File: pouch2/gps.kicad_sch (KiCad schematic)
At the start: 4 parts

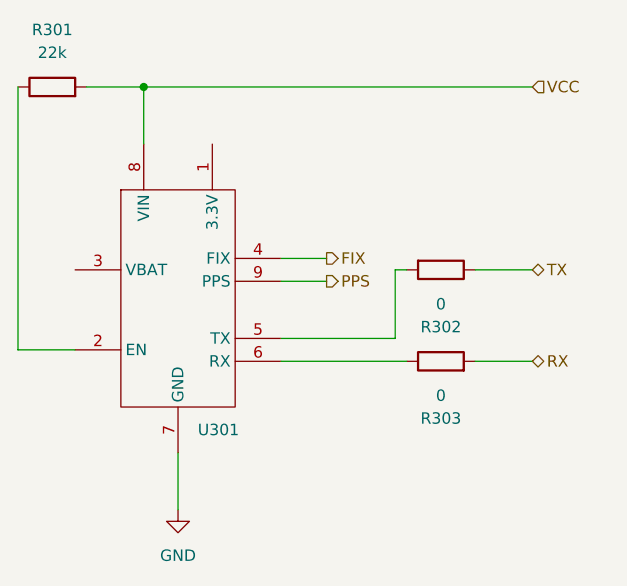
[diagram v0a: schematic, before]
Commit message: started routing
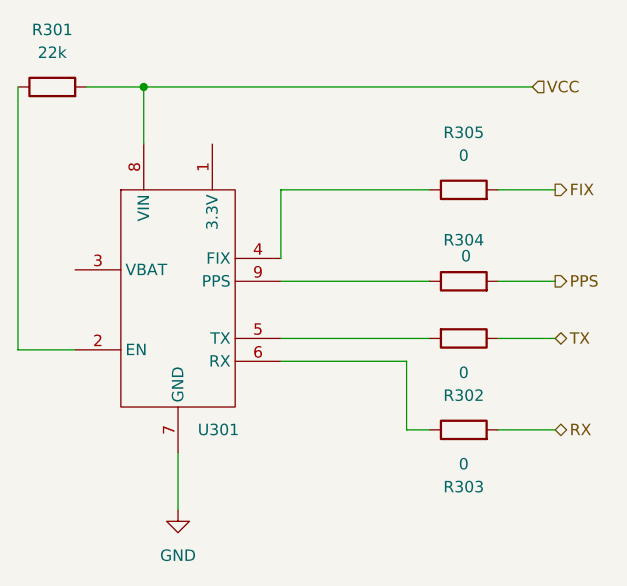
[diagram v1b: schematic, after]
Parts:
- added R304, R305: 0, Resistor_SMD:R_0805_2012Metric, symbol Device:R
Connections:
- net FIX: now also R305.2; no longer U301.4 (FIX)
- net PPS: now also R304.2; no longer U301.9 (PPS)
- new net: R304.1, U301.9 (PPS)
- new net: R305.1, U301.4 (FIX)
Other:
- moved on the sheet: R302, R303
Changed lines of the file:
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@@
-	(wire
-		(pts
-			(xy 182.88 67.31) (xy 182.88 74.93)
-		)
-		(stroke
-			(width 0)
-			(type default)
-		)
-	)
 	(wire
 		(pts
@@
 	(wire
 		(pts
+			(xy 184.15 77.47) (xy 170.18 77.47)
+		)
+		(stroke
+			(width 0)
+			(type default)
+		)
+	)
+	(wire
+		(pts
 			(xy 148.59 46.99) (xy 154.94 46.99)
 		)
@@
 	(wire
 		(pts
-			(xy 170.18 77.47) (xy 184.15 77.47)
-		)
-		(stroke
-			(width 0)
-			(type default)
-		)
-	)
-	(wire
-		(pts
-			(xy 170.18 68.58) (xy 175.26 68.58)
+			(xy 184.15 85.09) (xy 186.69 85.09)
+		)
+		(stroke
+			(width 0)
+			(type default)
+		)
+	)
+	(wire
+		(pts
+			(xy 170.18 68.58) (xy 186.69 68.58)
+		)
+		(stroke
+			(width 0)
+			(type default)
+		)
+	)
+	(wire
+		(pts
+			(xy 170.18 58.42) (xy 170.18 66.04)
 		)
 		(stroke
@@
 	(wire
 		(pts
-			(xy 198.12 67.31) (xy 191.77 67.31)
-		)
-		(stroke
-			(width 0)
-			(type default)
-		)
-	)
-	(wire
-		(pts
-			(xy 182.88 67.31) (xy 184.15 67.31)
-		)
-		(stroke
-			(width 0)
-			(type default)
-		)
-	)
-	(wire
-		(pts
-			(xy 170.18 66.04) (xy 175.26 66.04)
-		)
-		(stroke
-			(width 0)
-			(type default)
-		)
-	)
-	(wire
-		(pts
-			(xy 170.18 74.93) (xy 182.88 74.93)
-		)
-		(stroke
-			(width 0)
-			(type default)
-		)
-	)
-	(wire
-		(pts
-			(xy 198.12 77.47) (xy 191.77 77.47)
+			(xy 200.66 74.93) (xy 194.31 74.93)
+		)
+		(stroke
+			(width 0)
+			(type default)
+		)
+	)
+	(wire
+		(pts
+			(xy 194.31 58.42) (xy 200.66 58.42)
+		)
+		(stroke
+			(width 0)
+			(type default)
+		)
+	)
+	(wire
+		(pts
+			(xy 170.18 58.42) (xy 186.69 58.42)
+		)
+		(stroke
+			(width 0)
+			(type default)
+		)
+	)
+	(wire
+		(pts
+			(xy 170.18 74.93) (xy 186.69 74.93)
+		)
+		(stroke
+			(width 0)
+			(type default)
+		)
+	)
+	(wire
+		(pts
+			(xy 194.31 68.58) (xy 200.66 68.58)
+		)
+		(stroke
+			(width 0)
+			(type default)
+		)
+	)
+	(wire
+		(pts
+			(xy 184.15 85.09) (xy 184.15 77.47)
+		)
+		(stroke
+			(width 0)
+			(type default)
+		)
+	)
+	(wire
+		(pts
+			(xy 200.66 85.09) (xy 194.31 85.09)
 		)
 		(stroke
@@
 	(hierarchical_label "FIX"
 		(shape output)
-		(at 175.26 66.04 0)
+		(at 200.66 58.42 0)
 		(fields_autoplaced yes)
 		(effects
@@
 	(hierarchical_label "TX"
 		(shape bidirectional)
-		(at 198.12 67.31 0)
+		(at 200.66 74.93 0)
 		(fields_autoplaced yes)
 		(effects
@@
 	(hierarchical_label "RX"
 		(shape bidirectional)
-		(at 198.12 77.47 0)
+		(at 200.66 85.09 0)
 		(fields_autoplaced yes)
 		(effects
@@
 	(hierarchical_label "PPS"
 		(shape output)
-		(at 175.26 68.58 0)
+		(at 200.66 68.58 0)
 		(fields_autoplaced yes)
 		(effects
@@
 	(symbol
 		(lib_id "Device:R")
-		(at 187.96 67.31 270)
+		(at 190.5 74.93 270)
 		(unit 1)
 		(exclude_from_sim no)
@@
 		(fields_autoplaced yes)
 		(property "Reference" "R302"
-			(at 187.96 73.66 90)
+			(at 190.5 81.28 90)
 			(effects
 				(font
@@
 		)
 		(property "Value" "0"
-			(at 187.96 71.12 90)
+			(at 190.5 78.74 90)
 			(effects
 				(font
@@
 		)
 		(property "Footprint" "Resistor_SMD:R_0805_2012Metric"
-			(at 187.96 65.532 90)
+			(at 190.5 73.152 90)
 			(effects
 				(font
@@
 		)
 		(property "Datasheet" "~"
-			(at 187.96 67.31 0)
+			(at 190.5 74.93 0)
 			(effects
 				(font
@@
 		)
 		(property "Description" "Resistor"
-			(at 187.96 67.31 0)
+			(at 190.5 74.93 0)
 			(effects
 				(font
@@
 				(path "/278cfa6b-9496-4a22-b425-8abdb96793ef/d0ac005f-caac-4a17-bc1d-5f52781e91da"
 					(reference "R301")
+					(unit 1)
+				)
+			)
+		)
+	)
+	(symbol
+		(lib_id "Device:R")
+		(at 190.5 68.58 90)
+		(unit 1)
+		(exclude_from_sim no)
+		(in_bom yes)
+		(on_board yes)
+		(dnp no)
+		(property "Reference" "R304"
+			(at 190.5 64.008 90)
+			(effects
+				(font
+					(size 1.27 1.27)
+				)
+			)
+		)
+		(property "Value" "0"
+			(at 190.754 65.786 90)
+			(effects
+				(font
+					(size 1.27 1.27)
+				)
+			)
+		)
+		(property "Footprint" "Resistor_SMD:R_0805_2012Metric"
+			(at 190.5 70.358 90)
+			(effects
+				(font
+					(size 1.27 1.27)
+				)
+				(hide yes)
+			)
+		)
+		(property "Datasheet" "~"
+			(at 190.5 68.58 0)
+			(effects
+				(font
+					(size 1.27 1.27)
+				)
+				(hide yes)
+			)
+		)
+		(property "Description" "Resistor"
+			(at 190.5 68.58 0)
+			(effects
+				(font
+					(size 1.27 1.27)
+				)
+				(hide yes)
+			)
+		)
+		(pin "1"
+		)
+		(pin "2"
+		)
+		(instances
+			(project ""
+				(path "/278cfa6b-9496-4a22-b425-8abdb96793ef/d0ac005f-caac-4a17-bc1d-5f52781e91da"
+					(reference "R304")
+					(unit 1)
+				)
+			)
+		)
+	)
+	(symbol
+		(lib_id "Device:R")
+		(at 190.5 58.42 90)
+		(unit 1)
+		(exclude_from_sim no)
+		(in_bom yes)
+		(on_board yes)
+		(dnp no)
+		(fields_autoplaced yes)
+		(property "Reference" "R305"
+			(at 190.5 52.07 90)
+			(effects
+				(font
+					(size 1.27 1.27)
+				)
+			)
+		)
+		(property "Value" "0"
+			(at 190.5 54.61 90)
+			(effects
+				(font
+					(size 1.27 1.27)
+				)
+			)
+		)
+		(property "Footprint" "Resistor_SMD:R_0805_2012Metric"
+			(at 190.5 60.198 90)
+			(effects
+				(font
+					(size 1.27 1.27)
+				)
+				(hide yes)
+			)
+		)
+		(property "Datasheet" "~"
+			(at 190.5 58.42 0)
+			(effects
+				(font
+					(size 1.27 1.27)
+				)
+				(hide yes)
+			)
+		)
+		(property "Description" "Resistor"
+			(at 190.5 58.42 0)
+			(effects
+				(font
+					(size 1.27 1.27)
+				)
+				(hide yes)
+			)
+		)
+		(pin "1"
+		)
+		(pin "2"
+		)
+		(instances
+			(project ""
+				(path "/278cfa6b-9496-4a22-b425-8abdb96793ef/d0ac005f-caac-4a17-bc1d-5f52781e91da"
+					(reference "R305")
 					(unit 1)
 				)
@@
 	(symbol
 		(lib_id "Device:R")
-		(at 187.96 77.47 90)
+		(at 190.5 85.09 90)
 		(unit 1)
 		(exclude_from_sim no)
@@
 		(fields_autoplaced yes)
 		(property "Reference" "R303"
-			(at 187.96 83.82 90)
+			(at 190.5 91.44 90)
 			(effects
 				(font
@@
 		)
 		(property "Value" "0"
-			(at 187.96 81.28 90)
+			(at 190.5 88.9 90)
 			(effects
 				(font
@@
 		)
 		(property "Footprint" "Resistor_SMD:R_0805_2012Metric"
-			(at 187.96 79.248 90)
+			(at 190.5 86.868 90)
 			(effects
 				(font
@@
 		)
 		(property "Datasheet" "~"
-			(at 187.96 77.47 0)
+			(at 190.5 85.09 0)
 			(effects
 				(font
@@
 		)
 		(property "Description" "Resistor"
-			(at 187.96 77.47 0)
-			(effects
-				(font
+			(at 190.5 85.09 0)
+			(effects
+				(font
